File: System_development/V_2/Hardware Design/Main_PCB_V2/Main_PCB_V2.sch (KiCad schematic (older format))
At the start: 17 parts, among them J1 Conn_Coaxial, J2 Conn_Coaxial, J3 Conn_Coaxial, J4 Conn_Coaxial, J5 Conn_Coaxial, J6 Conn_Coaxial, J7 Conn_Coaxial, J8 Conn_Coaxial, U1 ADP-2-1W, U2 ADG901BRMZ, U3 ADE-6

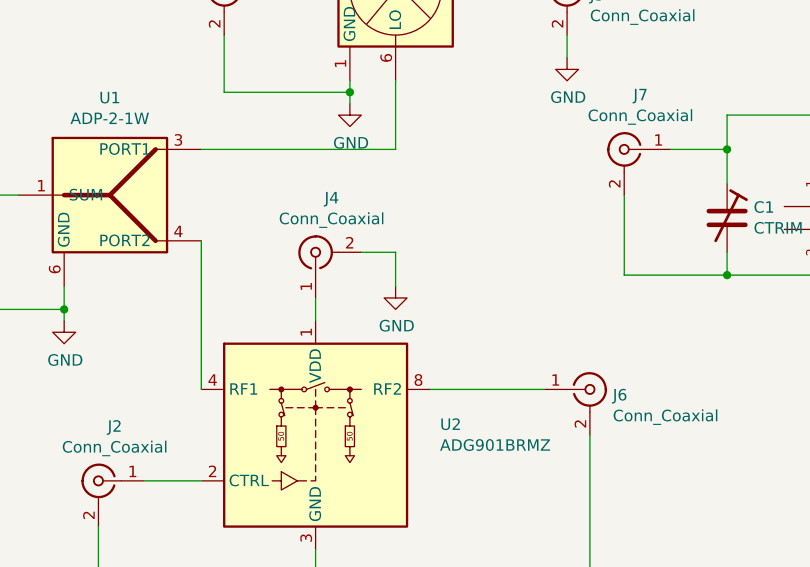
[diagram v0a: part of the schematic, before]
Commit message: Large update to V1 & V2 folders
Updated and added several folders
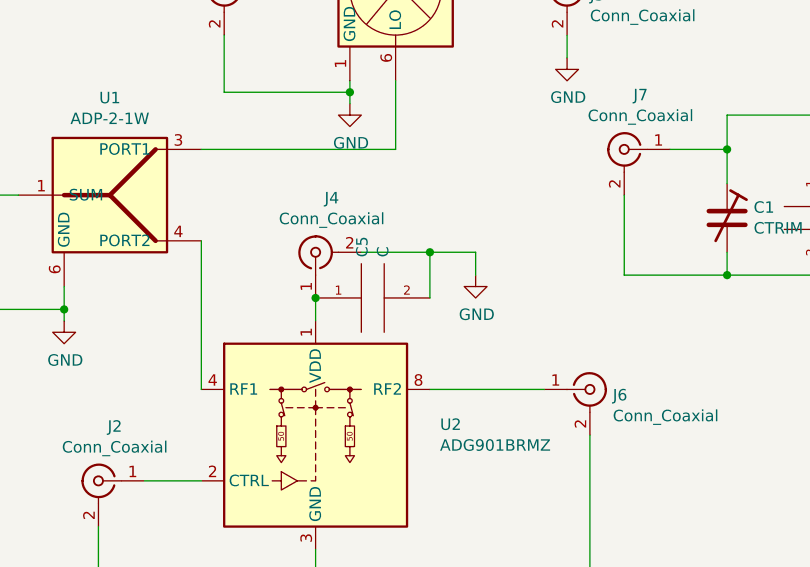
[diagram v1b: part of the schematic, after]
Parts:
- added C5: C, Capacitor_SMD:C_1210_3225Metric_Pad1.33x2.70mm_HandSolder, symbol pspice:C
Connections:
- net GND: now also C5.2
- net at J4.1 (In), U2.1 (VDD): now also C5.1
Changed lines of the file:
@@
 $EndComp
-Wire Wire Line
-	4650 2750 4650 2850
 Wire Wire Line
 	4150 2500 4150 3150
@@
 L power:GND #PWR04
 U 1 1 60DE8E11
-P 5000 2700
-F 0 "#PWR04" H 5000 2450 50  0001 C CNN
-F 1 "GND" H 5005 2527 50  0000 C CNN
-F 2 "" H 5000 2700 50  0001 C CNN
-F 3 "" H 5000 2700 50  0001 C CNN
-	1    5000 2700
-	1    0    0    -1
-$EndComp
-Wire Wire Line
-	4850 2550 5000 2550
-Wire Wire Line
-	5000 2550 5000 2700
+P 5350 2650
+F 0 "#PWR04" H 5350 2400 50  0001 C CNN
+F 1 "GND" H 5355 2477 50  0000 C CNN
+F 2 "" H 5350 2650 50  0001 C CNN
+F 3 "" H 5350 2650 50  0001 C CNN
+	1    5350 2650
+	1    0    0    -1
+$EndComp
 $Comp
 L Connector:Conn_Coaxial J5
@@
 	-1   0    0    1
 $EndComp
+Wire Wire Line
+	4650 2750 4650 2850
+$Comp
+L pspice:C C5
+U 1 1 60E4CBF7
+P 4900 2750
+F 0 "C5" H 5078 2796 50  0000 L CNN
+F 1 "C" H 5078 2705 50  0000 L CNN
+F 2 "Capacitor_SMD:C_1210_3225Metric_Pad1.33x2.70mm_HandSolder" H 4900 2750 50  0001 C CNN
+F 3 "~" H 4900 2750 50  0001 C CNN
+	1    4900 2750
+	0    -1   -1   0
+$EndComp
+Connection ~ 4650 2750
+Wire Wire Line
+	5350 2550 5350 2650
+Wire Wire Line
+	4850 2550 5150 2550
+Wire Wire Line
+	5150 2550 5150 2750
+Connection ~ 5150 2550
+Wire Wire Line
+	5150 2550 5350 2550
 $EndSCHEMATC
